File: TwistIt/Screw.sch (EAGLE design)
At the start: 6 parts

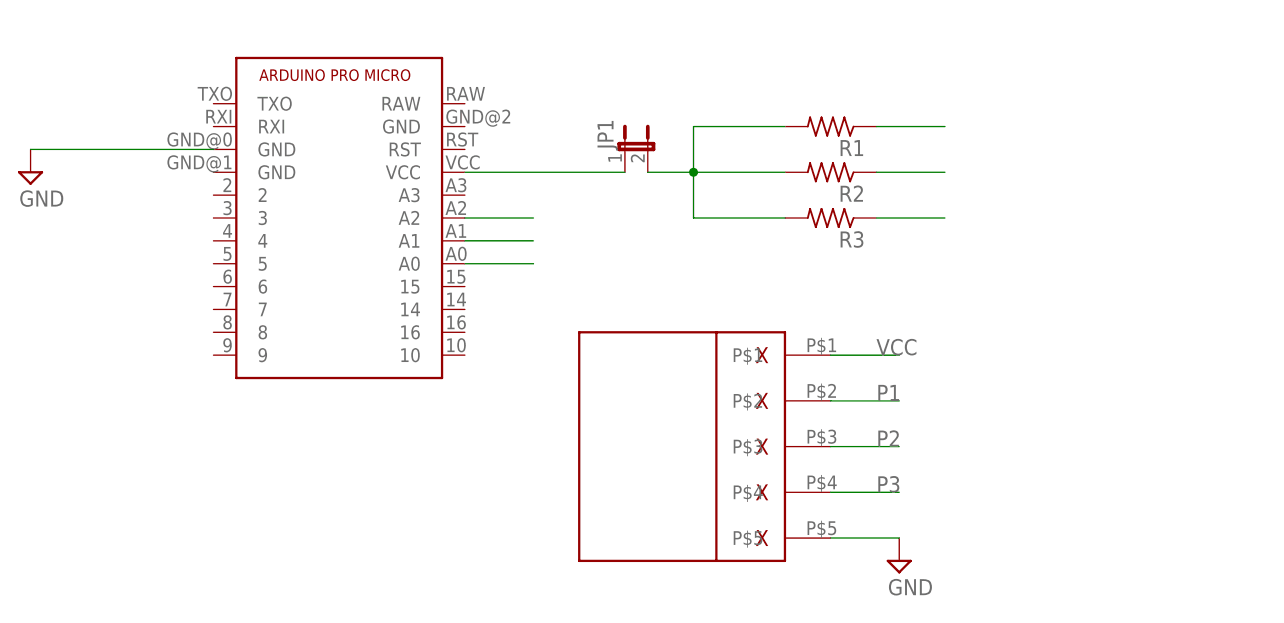
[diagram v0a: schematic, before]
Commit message: Minor fixes everywhere
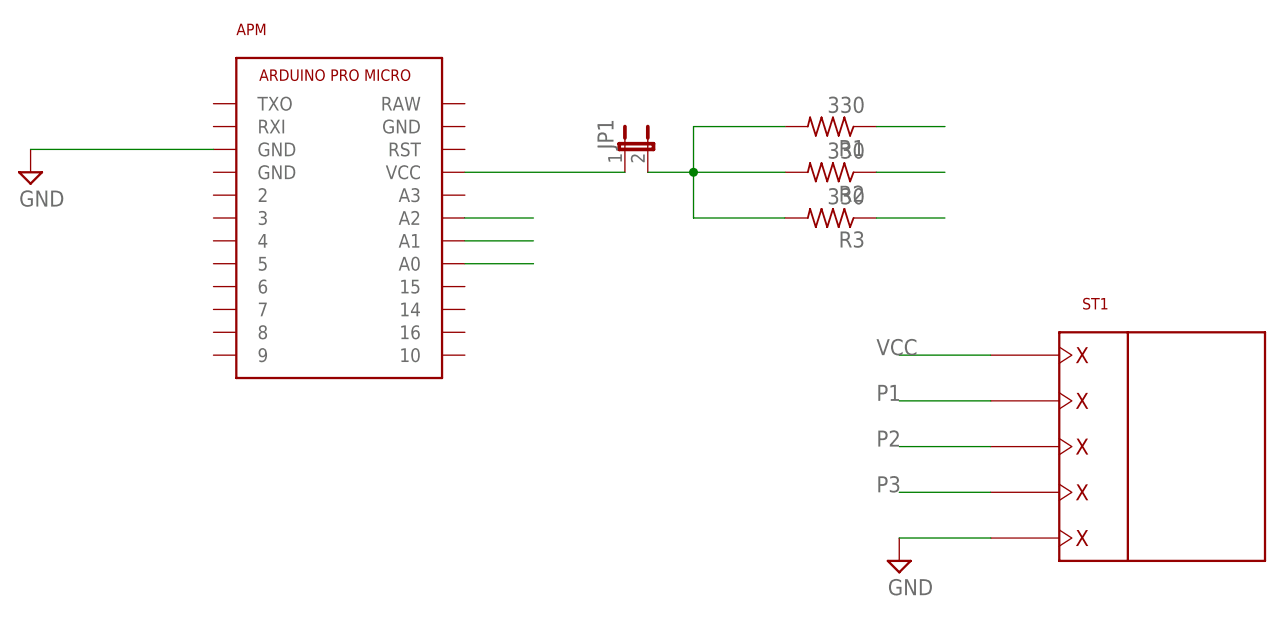
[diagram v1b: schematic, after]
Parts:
- removed U$2: 5PIN_SCREW, pie:5PIN_SCREW
- added ST1: (no value), pie:5PIN_SCREW
- R1, R2, R3: value (none) -> 330
- renumbered U$1 to APM
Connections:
- net GND: now also ST1.P$5; no longer U$2.P$5
- net P1: now also ST1.P$2; no longer U$2.P$2
- net P2: now also ST1.P$3; no longer U$2.P$3
- net P3: now also ST1.P$4; no longer U$2.P$4
- net VCC: now also ST1.P$1; no longer U$2.P$1
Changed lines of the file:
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@@
 </classes>
 <parts>
-<part name="U$1" library="pie" deviceset="ARDUINO_PRO_MICRO" device=""/>
-<part name="FRAME1" library="pie" deviceset="FRAME-LETTER" device="">
-<attribute name="REVISION" value="A"/>
+<part name="APM" library="pie" deviceset="ARDUINO_PRO_MICRO" device=""/>
+<part name="FRAME1" library="pie" deviceset="FRAME_SCHEMATIC" device="">
+<attribute name="AUTHOR" value="Mohammed Hossain, Seiya Ono"/>
+<attribute name="REVISION" value="9B"/>
 </part>
-<part name="R1" library="resistor" deviceset="R-US_" device="R0603"/>
-<part name="R2" library="resistor" deviceset="R-US_" device="R0603"/>
-<part name="R3" library="resistor" deviceset="R-US_" device="R0603"/>
+<part name="R1" library="resistor" deviceset="R-US_" device="R0603" value="330"/>
+<part name="R2" library="resistor" deviceset="R-US_" device="R0603" value="330"/>
+<part name="R3" library="resistor" deviceset="R-US_" device="R0603" value="330"/>
 <part name="SUPPLY2" library="pie" deviceset="GND" device=""/>
 <part name="JP1" library="jumper" deviceset="JP1E" device=""/>
-<part name="U$2" library="pie" deviceset="5PIN_SCREW" device=""/>
+<part name="ST1" library="pie" deviceset="5PIN_SCREW" device=""/>
 <part name="SUPPLY1" library="pie" deviceset="GND" device=""/>
 </parts>
@@
 </plain>
 <instances>
-<instance part="U$1" gate="G$1" x="60.96" y="93.98"/>
-<instance part="FRAME1" gate="G$1" x="0" y="0"/>
+<instance part="APM" gate="G$1" x="60.96" y="93.98"/>
+<instance part="FRAME1" gate="G$1" x="0" y="0">
+<attribute name="AUTHOR" x="0" y="0" size="1.778" layer="96" display="off"/>
+</instance>
 <instance part="FRAME1" gate="G$2" x="147.32" y="0">
 <attribute name="REVISION" x="147.32" y="0" size="1.778" layer="96"/>
@@
 <instance part="SUPPLY2" gate="GND" x="27.94" y="99.06"/>
 <instance part="JP1" gate="A" x="93.98" y="101.6"/>
-<instance part="U$2" gate="G$1" x="101.6" y="71.12" rot="R180"/>
+<instance part="ST1" gate="G$1" x="154.94" y="68.58"/>
 <instance part="SUPPLY1" gate="GND" x="124.46" y="55.88"/>
 </instances>
@@
 <segment>
 <pinref part="SUPPLY2" gate="GND" pin="GND"/>
-<pinref part="U$1" gate="G$1" pin="GND@0"/>
+<pinref part="APM" gate="G$1" pin="GND@0"/>
 <wire x1="27.94" y1="101.6" x2="48.26" y2="101.6" width="0.1524" layer="91"/>
 </segment>
 <segment>
-<pinref part="U$2" gate="G$1" pin="P$5"/>
-<wire x1="116.84" y1="58.42" x2="124.46" y2="58.42" width="0.1524" layer="91"/>
+<pinref part="ST1" gate="G$1" pin="P$5"/>
+<wire x1="134.62" y1="58.42" x2="124.46" y2="58.42" width="0.1524" layer="91"/>
 <pinref part="SUPPLY1" gate="GND" pin="GND"/>
 </segment>
@@
 </segment>
 <segment>
-<pinref part="U$2" gate="G$1" pin="P$2"/>
-<wire x1="116.84" y1="73.66" x2="124.46" y2="73.66" width="0.1524" layer="91"/>
+<pinref part="ST1" gate="G$1" pin="P$2"/>
+<wire x1="134.62" y1="73.66" x2="124.46" y2="73.66" width="0.1524" layer="91"/>
 <label x="121.92" y="73.66" size="1.778" layer="95"/>
 </segment>
 <segment>
-<pinref part="U$1" gate="G$1" pin="A2"/>
+<pinref part="APM" gate="G$1" pin="A2"/>
 <wire x1="76.2" y1="93.98" x2="83.82" y2="93.98" width="0.1524" layer="91"/>
 </segment>
@@
 <net name="VCC" class="0">
 <segment>
-<pinref part="U$2" gate="G$1" pin="P$1"/>
-<wire x1="116.84" y1="78.74" x2="124.46" y2="78.74" width="0.1524" layer="91"/>
+<pinref part="ST1" gate="G$1" pin="P$1"/>
+<wire x1="134.62" y1="78.74" x2="124.46" y2="78.74" width="0.1524" layer="91"/>
 <label x="121.92" y="78.74" size="1.778" layer="95"/>
 </segment>
 <segment>
 <pinref part="JP1" gate="A" pin="1"/>
-<pinref part="U$1" gate="G$1" pin="VCC"/>
+<pinref part="APM" gate="G$1" pin="VCC"/>
 <wire x1="76.2" y1="99.06" x2="93.98" y2="99.06" width="0.1524" layer="91"/>
 </segment>
@@
 <net name="P2" class="0">
 <segment>
-<pinref part="U$2" gate="G$1" pin="P$3"/>
-<wire x1="116.84" y1="68.58" x2="124.46" y2="68.58" width="0.1524" layer="91"/>
+<pinref part="ST1" gate="G$1" pin="P$3"/>
+<wire x1="134.62" y1="68.58" x2="124.46" y2="68.58" width="0.1524" layer="91"/>
 <label x="121.92" y="68.58" size="1.778" layer="95"/>
 </segment>
 <segment>
-<pinref part="U$1" gate="G$1" pin="A1"/>
+<pinref part="APM" gate="G$1" pin="A1"/>
 <wire x1="76.2" y1="91.44" x2="83.82" y2="91.44" width="0.1524" layer="91"/>
 </segment>
@@
 <net name="P3" class="0">
 <segment>
-<pinref part="U$2" gate="G$1" pin="P$4"/>
-<wire x1="116.84" y1="63.5" x2="124.46" y2="63.5" width="0.1524" layer="91"/>
+<pinref part="ST1" gate="G$1" pin="P$4"/>
+<wire x1="134.62" y1="63.5" x2="124.46" y2="63.5" width="0.1524" layer="91"/>
 <label x="121.92" y="63.5" size="1.778" layer="95"/>
 </segment>
 <segment>
-<pinref part="U$1" gate="G$1" pin="A0"/>
+<pinref part="APM" gate="G$1" pin="A0"/>
 <wire x1="76.2" y1="88.9" x2="83.82" y2="88.9" width="0.1524" layer="91"/>
 </segment>
